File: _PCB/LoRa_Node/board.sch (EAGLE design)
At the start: 26 parts

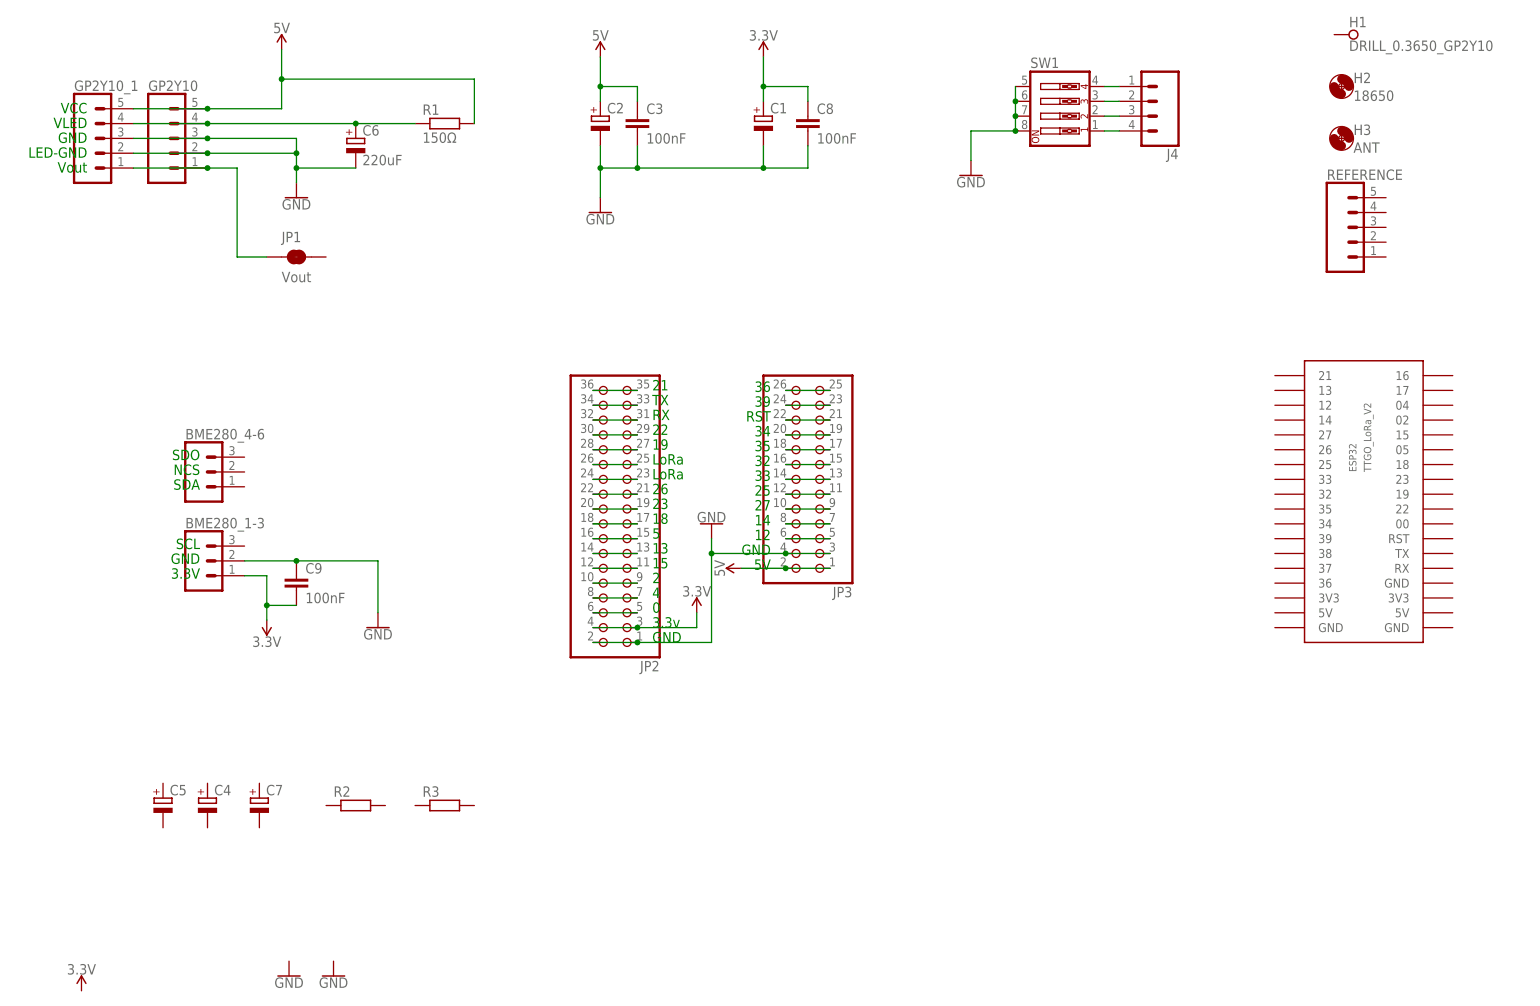
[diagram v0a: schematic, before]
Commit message: LoRa update
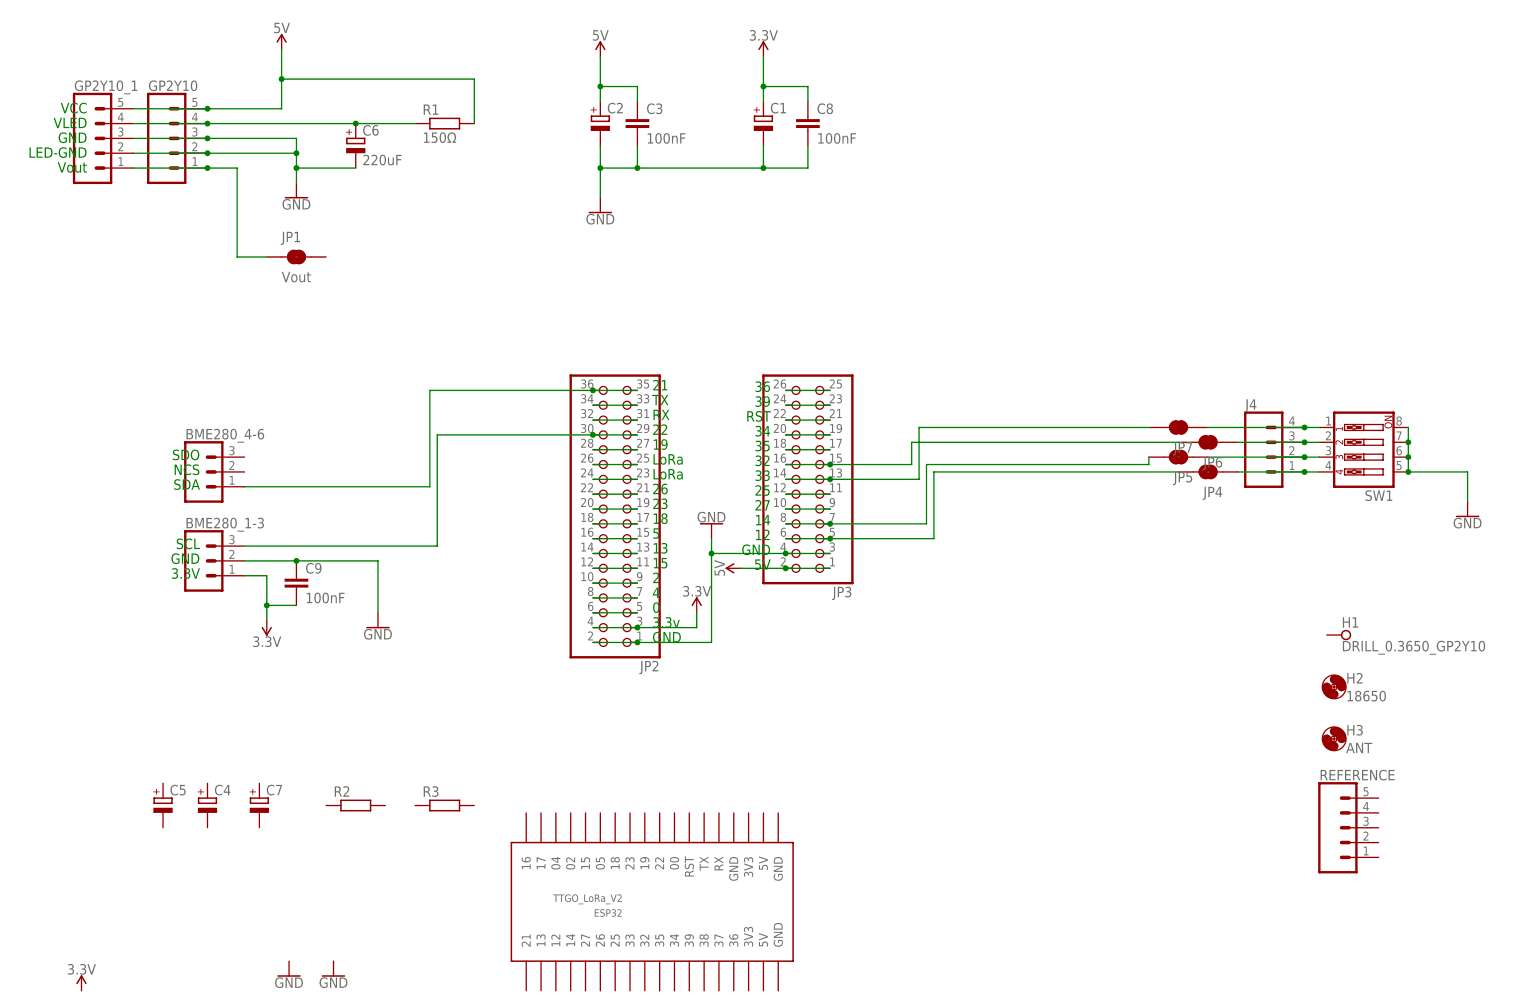
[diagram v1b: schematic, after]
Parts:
- added JP4, JP5, JP6, JP7: JUMPER-SMT_2_NC_TRACE_SILK, SparkFun-Jumpers:JUMPER-SMT_2_NC_TRACE_SILK
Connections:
- net N$14: now also JP6.2
- net N$15: now also JP7.2
- net N$18: now also JP5.2
- net N$19: now also JP4.2
- net N$3: now also BME280_4-6.1
- net N$39: now also JP4.1
- net N$40: now also JP5.1
- net N$41: now also JP6.1
- net N$42: now also JP7.1
- net N$6: now also BME280_1-3.3
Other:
- moved on the sheet: ESP32, H1, H2, H3, J4, REFERENCE, SW1
